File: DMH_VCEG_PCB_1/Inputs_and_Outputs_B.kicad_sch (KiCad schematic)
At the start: 13 parts, among them J11 TS_Jack_6.35mm_Sw, J12 TS_Jack_6.35mm_Sw, J13 TS_Jack_6.35mm_Sw, J14 TS_Jack_6.35mm_Sw, J15 TS_Jack_6.35mm_Sw, J16 TS_Jack_6.35mm_Sw, J17 TS_Jack_6.35mm_Sw, J18 TS_Jack_6.35mm_Sw, J19 TS_Jack_6.35mm_Sw, J20 TS_Jack_6.35mm_Sw, J201 IDC_02x05, J51 Conn_01x06, J61 Conn_01x06

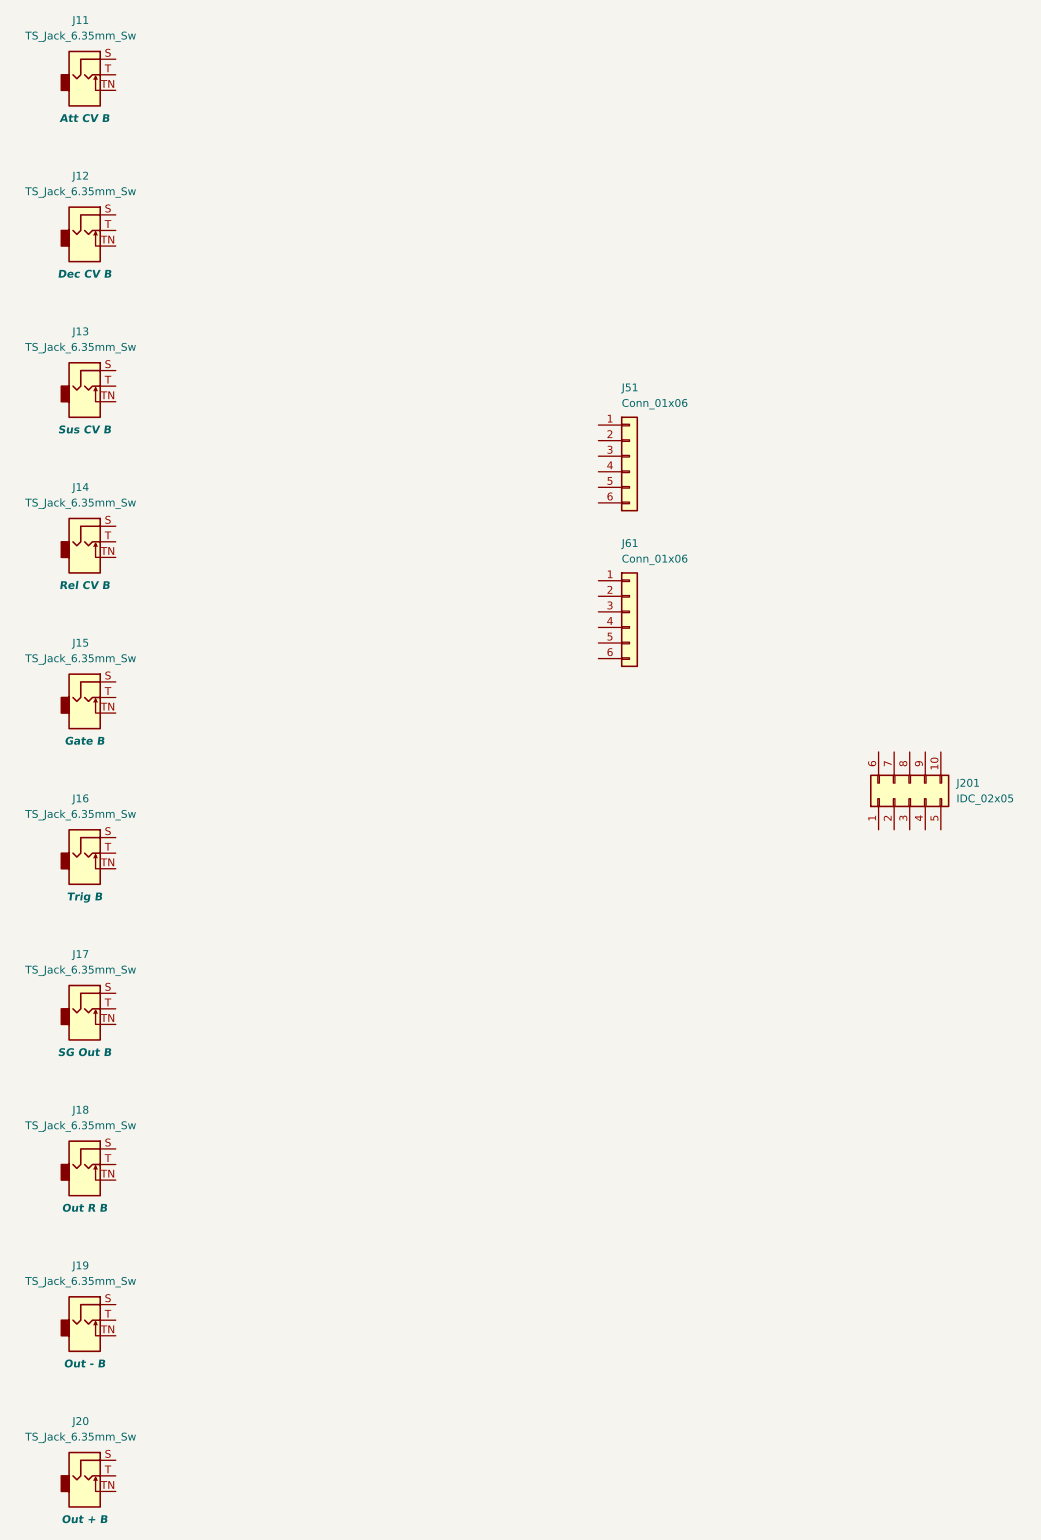
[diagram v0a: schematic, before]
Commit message: IO pages done
Core Circuit A ongoing
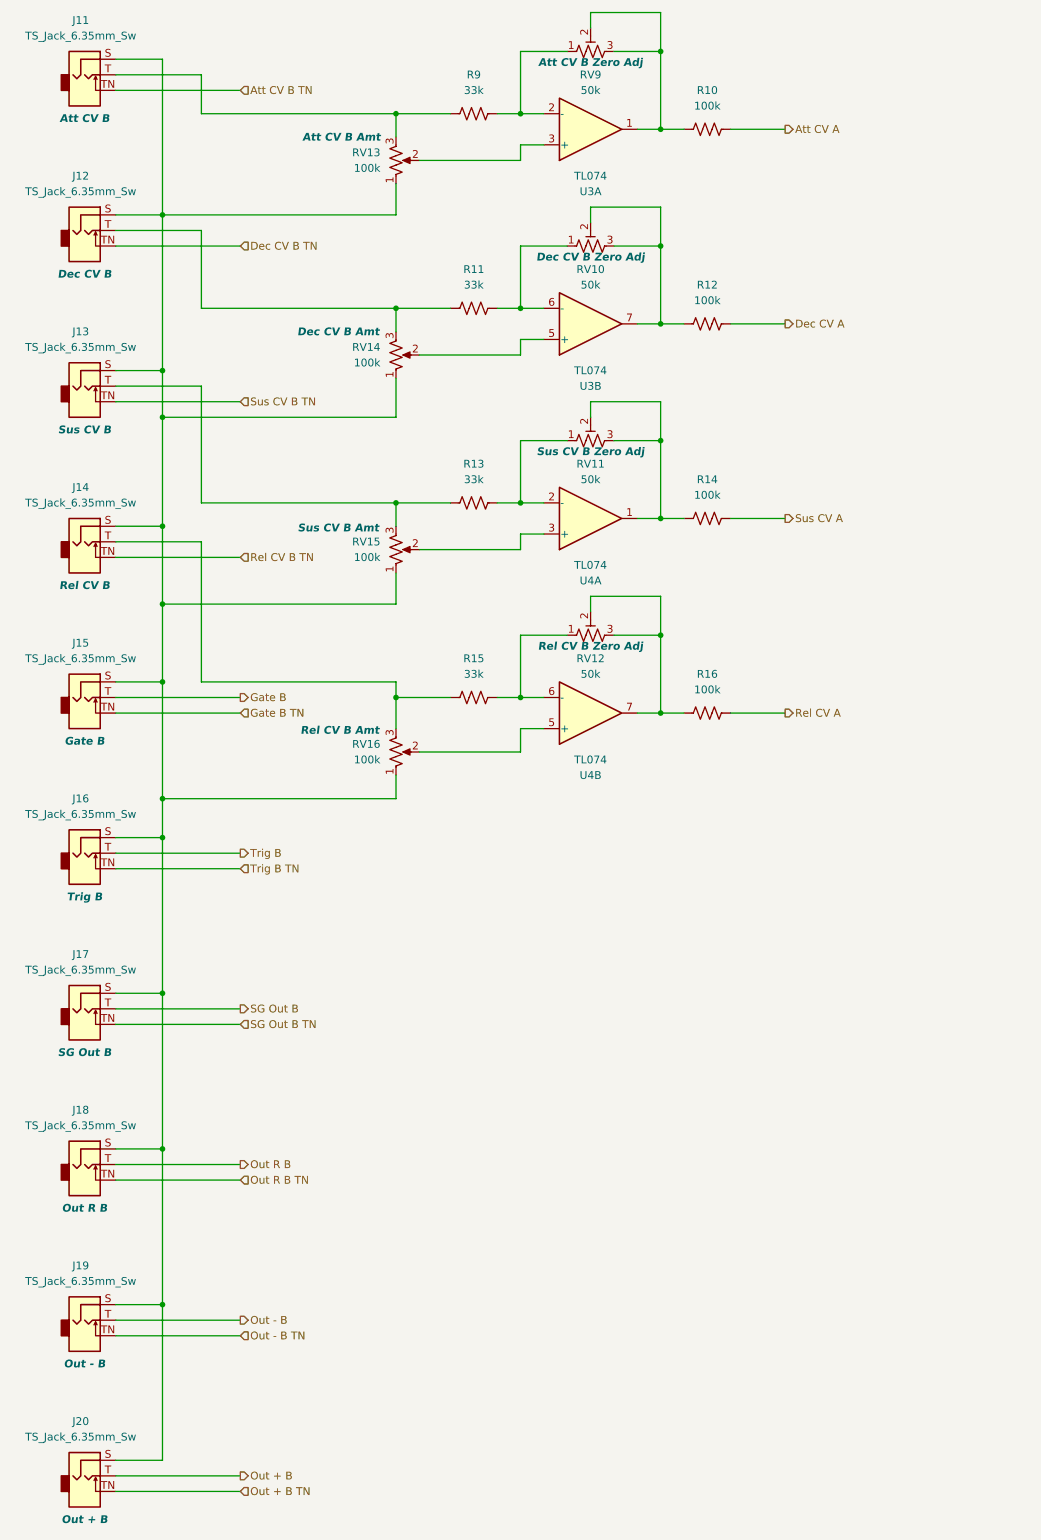
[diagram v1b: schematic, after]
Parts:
- removed J201: IDC_02x05, SynthStuff:IDC-Header_2x05_P2.54mm_Vertical_BackBone, symbol SynthStuff:BackBone_Connector_10Pin
- removed J51, J61: Conn_01x06, Connector_PinSocket_2.54mm:PinSocket_1x06_P2.54mm_Vertical, symbol Connector_Generic:Conn_01x06
- added R10, R12, R14, R16: 100k, Resistor_THT:R_Axial_DIN0207_L6.3mm_D2.5mm_P7.62mm_Horizontal, symbol Device:R_US
- added R11, R13, R15, R9: 33k, Resistor_THT:R_Axial_DIN0207_L6.3mm_D2.5mm_P7.62mm_Horizontal, symbol Device:R_US
- added RV10, RV11, RV12, RV9: 50k, Potentiometer_THT:Potentiometer_Bourns_3296W_Vertical, symbol Device:R_Potentiometer_Trim_US
- added RV13, RV14, RV15, RV16: 100k, SynthStuff:Potentiometer_TT_P110KH1, symbol Device:R_Potentiometer_US
- added U3, U4: TL074, Package_DIP:DIP-14_W7.62mm_Socket, symbol Amplifier_Operational:TL074
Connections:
- net at J14.S: now also J11.S, J12.S, J13.S, J15.S, J16.S, J17.S, J18.S, J19.S, J20.S, RV13.1, RV14.1, RV15.1, RV16.1
- net at J14.T: now also R15.1, RV16.3
- net Rel CV B TN: now reaches J14.TN
- net Out R B: now reaches J18.T
- net Out R B TN: now reaches J18.TN
- net Gate B: now reaches J15.T
- net Gate B TN: now reaches J15.TN
- net at J12.T: now also R11.1, RV14.3
- net Dec CV B TN: now reaches J12.TN
- net Out - B: now reaches J19.T
- net Out - B TN: now reaches J19.TN
- net at J11.T: now also R9.1, RV13.3
- net Att CV B TN: now reaches J11.TN
- net Trig B: now reaches J16.T
- net Trig B TN: now reaches J16.TN
- net at J13.T: now also R13.1, RV15.3
- net Sus CV B TN: now reaches J13.TN
- net Out + B: now reaches J20.T
- net Out + B TN: now reaches J20.TN
- net SG Out B: now reaches J17.T
- net SG Out B TN: now reaches J17.TN
- new net: R13.2, RV11.1, U4.2 (-)
- new net: R14.1, RV11.2, RV11.3, U4.1
- new net: R11.2, RV10.1, U3.6 (-)
- new net: R10.1, RV9.2, RV9.3, U3.1
- new net: R9.2, RV9.1, U3.2 (-)
- new net: RV13.2, U3.3 (+)
- new net: RV14.2, U3.5 (+)
- new net: R15.2, RV12.1, U4.6 (-)
- new net: R12.1, RV10.2, RV10.3, U3.7
- new net: RV16.2, U4.5 (+)
- new net: R16.1, RV12.2, RV12.3, U4.7
- new net: RV15.2, U4.3 (+)
- new net Att CV A: R10.2
- new net Dec CV A: R12.2
- new net Rel CV A: R16.2
- new net Sus CV A: R14.2
